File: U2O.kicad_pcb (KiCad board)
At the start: 2 copper layers, 28 x 27 mm, 21 parts, among them J1 AFBR-1624Z, J2 USB_B_Micro, J3 AFBR-2624Z, U1 CP2102N-Axx-xQFN20

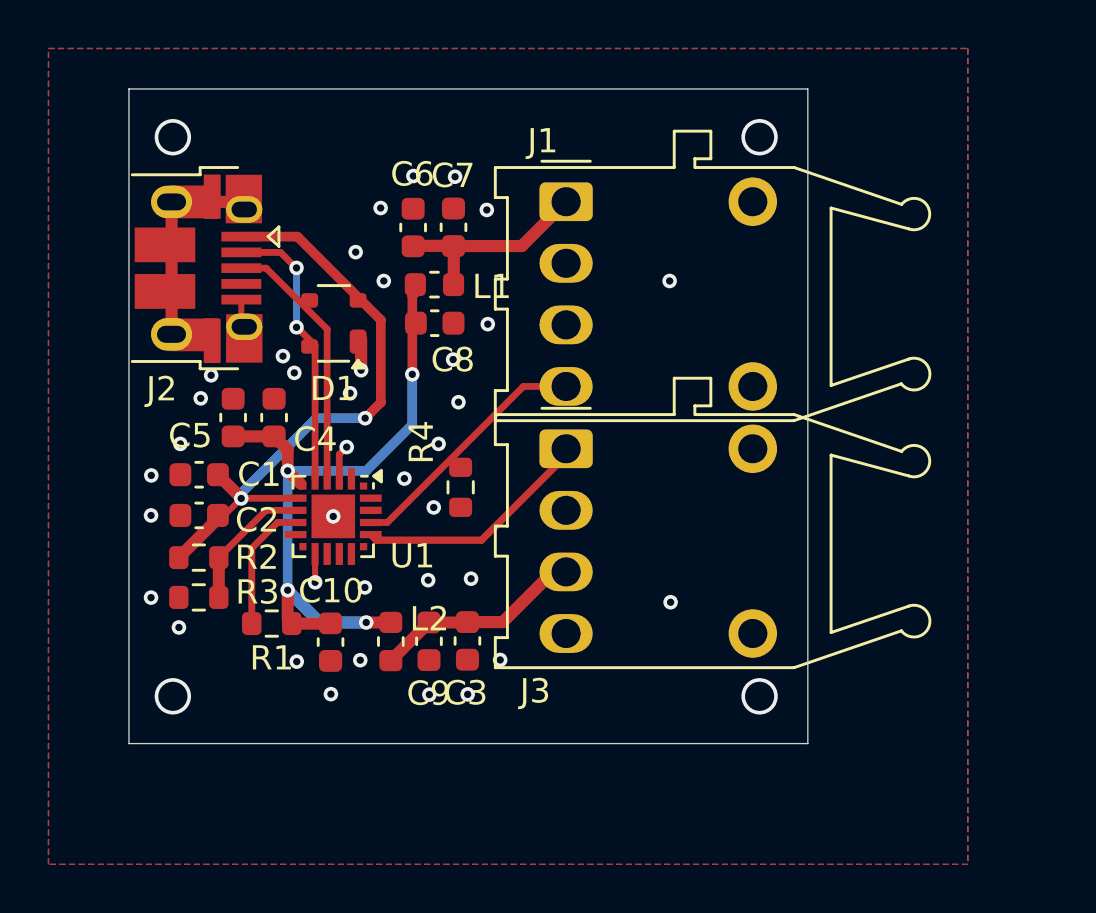
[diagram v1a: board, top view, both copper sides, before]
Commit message: final push
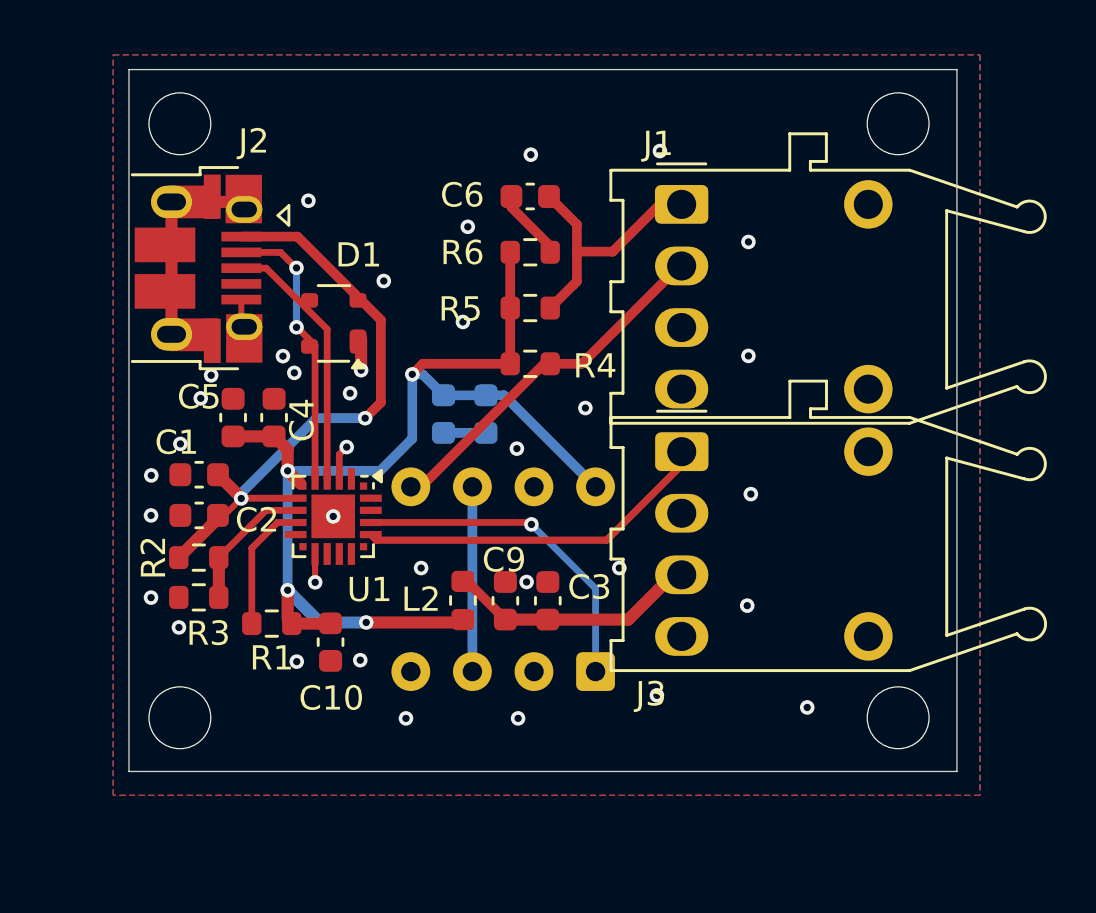
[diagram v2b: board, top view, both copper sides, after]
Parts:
- removed C7, C8: 10u, Capacitor_SMD:C_0603_1608Metric
- removed L1: 1u, Inductor_SMD:L_0603_1608Metric
- added C11: 100n, Capacitor_SMD:C_0603_1608Metric, B.Cu at (31.2, 29.8)
- added C12: 10u, Capacitor_SMD:C_0603_1608Metric, B.Cu at (33.0, 29.8)
- added R5: 100, Resistor_SMD:R_0603_1608Metric, F.Cu at (34.8, 25.4)
- added R6: 15, Resistor_SMD:R_0603_1608Metric, F.Cu at (34.8, 23.1)
- added U2: SN75454B, Package_DIP:DIP-8_W7.62mm, B.Cu at (37.5, 40.4)
- C6: value 100n -> 120p
- J1: value AFBR-1624Z -> AFBR-1528CZ
- R4: value 4.7K -> 2K
- moved R4 5.85 mm to (34.8, 27.7), turned to 0 degrees
- moved C6 5.00 mm to (34.8, 20.8), turned to 180 degrees
- moved J3 4.77 mm to (41.0, 31.3)
- moved J1 4.77 mm to (41.0, 21.1)
- moved C3 3.71 mm to (35.5, 37.5), turned to -90 degrees
- moved C9 3.57 mm to (33.8, 37.5), turned to -90 degrees
- moved L2 3.42 mm to (32.0, 37.4), turned to -90 degrees
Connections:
- C6 pad 1: GND -> Net-(J1-A)
- C6 pad 2: Net-(J1-VCCT) -> Net-(C6-Pad2)
- J1 pad 1: Net-(J1-VCCT) -> Net-(J1-A)
- J1 pad 2: unconnected-(J1-NC-Pad2) -> Net-(J1-K)
- J1 pad 4: TXD -> GND
- R4 pad 1: TXD -> VCC
- R4 pad 2: GND -> Net-(J1-K)
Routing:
- net VCC: track 28.5 -> 46.7 mm
- net Net-(J1-K): track 0.00 -> 15.1 mm
- net Net-(J1-A): track 0.00 -> 10.7 mm
- net Net-(J1-VCCT): track 8.68 -> 0.00 mm
- net Net-(U2-1Y): track 0.00 -> 7.62 mm
- net RXD: track 9.88 -> 14.8 mm
- net TXD: track 10.4 -> 13.8 mm, vias 0 -> 1
- net Net-(C6-Pad2): track 0.00 -> 2.96 mm
- net Net-(J3-VCCR): track 8.75 -> 11.6 mm
- net GND: track 14.6 -> 16.3 mm, vias 37 -> 35
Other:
- board size 28 x 27 mm -> 34.1 x 29 mm
